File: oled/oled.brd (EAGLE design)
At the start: 35.9 x 35.5 mm, 3 parts

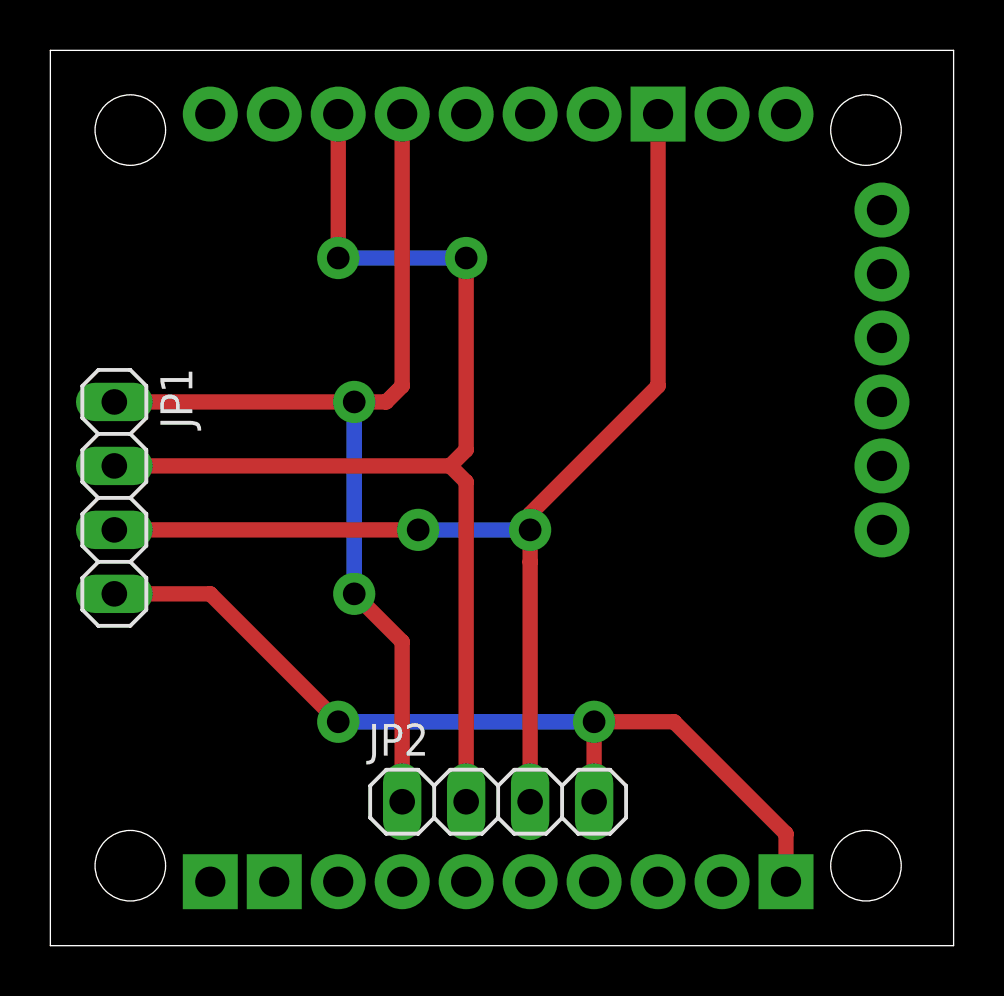
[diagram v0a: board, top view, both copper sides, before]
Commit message: Improve oled board
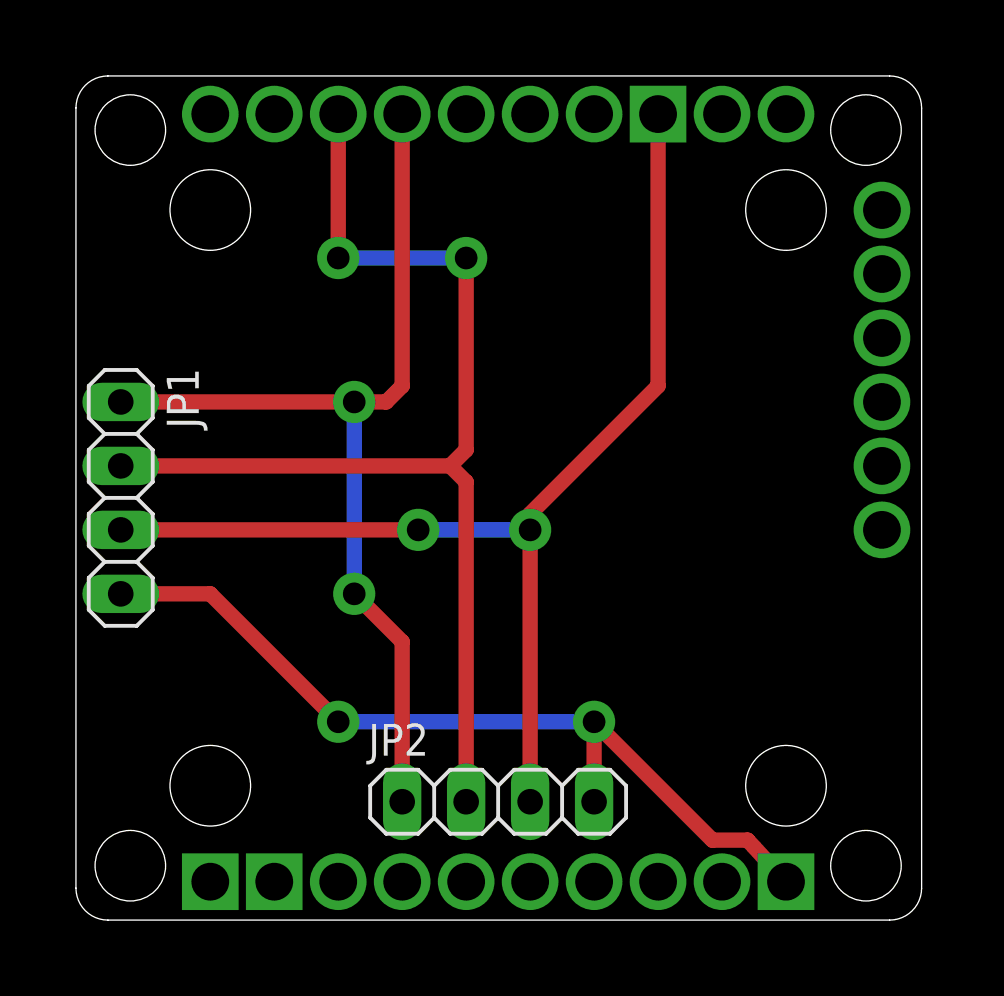
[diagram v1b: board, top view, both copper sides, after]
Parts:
- moved JP1 0.25 mm to (2.79, 17.8)
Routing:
- net +3V3: track 35.7 -> 34.4 mm
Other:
- board size 35.9 x 35.5 mm -> 33.6 x 33.5 mm
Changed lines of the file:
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@@
 <setting verticaltext="up"/>
 </settings>
-<grid distance="0.1" unitdist="inch" unit="inch" style="lines" multiple="1" display="yes" altdistance="0.025" altunitdist="inch" altunit="inch"/>
+<grid distance="0.05" unitdist="inch" unit="inch" style="lines" multiple="1" display="yes" altdistance="0.005" altunitdist="inch" altunit="inch"/>
 <layers>
 <layer number="1" name="Top" color="4" fill="1" visible="yes" active="yes"/>
@@
 <layer number="48" name="Document" color="7" fill="1" visible="yes" active="yes"/>
 <layer number="49" name="Reference" color="7" fill="1" visible="yes" active="yes"/>
+<layer number="50" name="dxf" color="7" fill="1" visible="no" active="no"/>
 <layer number="51" name="tDocu" color="7" fill="1" visible="yes" active="yes"/>
 <layer number="52" name="bDocu" color="7" fill="1" visible="yes" active="yes"/>
+<layer number="53" name="tGND_GNDA" color="7" fill="9" visible="no" active="no"/>
+<layer number="54" name="bGND_GNDA" color="1" fill="9" visible="no" active="no"/>
+<layer number="56" name="wert" color="7" fill="1" visible="no" active="no"/>
 <layer number="90" name="Modules" color="5" fill="1" visible="no" active="no"/>
 <layer number="91" name="Nets" color="2" fill="1" visible="no" active="no"/>
@@
 <layer number="97" name="Info" color="7" fill="1" visible="no" active="no"/>
 <layer number="98" name="Guide" color="6" fill="1" visible="no" active="no"/>
+<layer number="100" name="Muster" color="7" fill="1" visible="no" active="no"/>
+<layer number="101" name="Patch_Top" color="12" fill="4" visible="yes" active="yes"/>
+<layer number="102" name="Vscore" color="7" fill="1" visible="yes" active="yes"/>
+<layer number="103" name="tMap" color="7" fill="1" visible="yes" active="yes"/>
+<layer number="104" name="Name" color="7" fill="1" visible="yes" active="yes"/>
+<layer number="105" name="tPlate" color="7" fill="1" visible="yes" active="yes"/>
+<layer number="106" name="bPlate" color="7" fill="1" visible="yes" active="yes"/>
+<layer number="107" name="Crop" color="7" fill="1" visible="yes" active="yes"/>
+<layer number="116" name="Patch_BOT" color="9" fill="4" visible="yes" active="yes"/>
+<layer number="121" name="_tsilk" color="7" fill="1" visible="yes" active="yes"/>
+<layer number="122" name="_bsilk" color="7" fill="1" visible="yes" active="yes"/>
+<layer number="125" name="_tNames" color="7" fill="1" visible="yes" active="yes"/>
+<layer number="144" name="Drill_legend" color="7" fill="1" visible="yes" active="yes"/>
+<layer number="151" name="HeatSink" color="7" fill="1" visible="yes" active="yes"/>
+<layer number="200" name="200bmp" color="1" fill="10" visible="yes" active="yes"/>
+<layer number="201" name="201bmp" color="2" fill="1" visible="no" active="no"/>
+<layer number="202" name="202bmp" color="3" fill="1" visible="no" active="no"/>
+<layer number="203" name="203bmp" color="4" fill="10" visible="yes" active="yes"/>
+<layer number="204" name="204bmp" color="5" fill="10" visible="yes" active="yes"/>
+<layer number="205" name="205bmp" color="6" fill="10" visible="yes" active="yes"/>
+<layer number="206" name="206bmp" color="7" fill="10" visible="yes" active="yes"/>
+<layer number="207" name="207bmp" color="8" fill="10" visible="yes" active="yes"/>
+<layer number="208" name="208bmp" color="9" fill="10" visible="yes" active="yes"/>
+<layer number="209" name="209bmp" color="7" fill="1" visible="yes" active="yes"/>
+<layer number="210" name="210bmp" color="7" fill="1" visible="yes" active="yes"/>
+<layer number="211" name="211bmp" color="7" fill="1" visible="yes" active="yes"/>
+<layer number="212" name="212bmp" color="7" fill="1" visible="yes" active="yes"/>
+<layer number="213" name="213bmp" color="7" fill="1" visible="yes" active="yes"/>
+<layer number="214" name="214bmp" color="7" fill="1" visible="yes" active="yes"/>
+<layer number="215" name="215bmp" color="7" fill="1" visible="yes" active="yes"/>
+<layer number="216" name="216bmp" color="7" fill="1" visible="yes" active="yes"/>
+<layer number="250" name="Descript" color="3" fill="1" visible="no" active="no"/>
+<layer number="251" name="SMDround" color="12" fill="11" visible="no" active="no"/>
+<layer number="254" name="cooling" color="7" fill="1" visible="yes" active="yes"/>
 </layers>
 <board>
 <plain>
-<wire x1="0" y1="0" x2="35.865" y2="0" width="0" layer="20"/>
-<wire x1="35.865" y1="0" x2="35.865" y2="35.55" width="0" layer="20"/>
-<wire x1="35.865" y1="35.55" x2="0" y2="35.55" width="0" layer="20"/>
-<wire x1="0" y1="35.55" x2="0" y2="0" width="0" layer="20"/>
+<wire x1="2.286" y1="1.016" x2="33.325" y2="1.016" width="0" layer="20"/>
+<wire x1="33.325" y1="1.016" x2="34.595" y2="2.286" width="0" layer="20" curve="90"/>
+<wire x1="34.595" y1="2.286" x2="34.595" y2="33.264" width="0" layer="20"/>
+<wire x1="34.595" y1="33.264" x2="33.325" y2="34.534" width="0" layer="20" curve="90"/>
+<wire x1="33.325" y1="34.534" x2="2.286" y2="34.534" width="0" layer="20"/>
+<wire x1="2.286" y1="34.534" x2="1.016" y2="33.264" width="0" layer="20" curve="90"/>
+<wire x1="1.016" y1="33.264" x2="1.016" y2="2.286" width="0" layer="20"/>
+<wire x1="1.016" y1="2.286" x2="2.286" y2="1.016" width="0" layer="20" curve="90"/>
+<hole x="29.21" y="6.35" drill="3.2"/>
+<hole x="6.35" y="6.35" drill="3.2"/>
+<hole x="29.21" y="29.21" drill="3.2"/>
+<hole x="6.35" y="29.21" drill="3.2"/>
 </plain>
 <attributes>
@@
 <elements>
 <element name="OLED/I2C" library="ESPstack" package="ESP-BOARD" value="ESP-BOARD" x="24.13" y="19.05"/>
-<element name="JP1" library="pinhead" package="1X04" value="" x="2.54" y="17.78" rot="R270"/>
+<element name="JP1" library="pinhead" package="1X04" value="" x="2.794" y="17.78" rot="R270"/>
 <element name="JP2" library="pinhead" package="1X04" value="" x="17.78" y="5.715"/>
 </elements>
@@
 <contactref element="JP1" pad="4"/>
 <contactref element="JP2" pad="4"/>
-<wire x1="2.54" y1="13.97" x2="6.35" y2="13.97" width="0.6096" layer="1"/>
+<wire x1="2.794" y1="13.97" x2="6.35" y2="13.97" width="0.6096" layer="1"/>
 <wire x1="6.35" y1="13.97" x2="11.43" y2="8.89" width="0.6096" layer="1"/>
 <via x="11.43" y="8.89" extent="1-16" drill="0.9" diameter="1.6764"/>
@@
 <via x="21.59" y="8.89" extent="1-16" drill="0.9" diameter="1.6764"/>
 <wire x1="21.59" y1="8.89" x2="21.59" y2="5.715" width="0.6096" layer="1"/>
-<wire x1="29.21" y1="2.54" x2="29.21" y2="4.445" width="0.6096" layer="1"/>
-<wire x1="29.21" y1="4.445" x2="24.765" y2="8.89" width="0.6096" layer="1"/>
-<wire x1="24.765" y1="8.89" x2="21.59" y2="8.89" width="0.6096" layer="1"/>
+<wire x1="29.21" y1="2.54" x2="27.686" y2="4.191" width="0.6096" layer="1"/>
+<wire x1="27.686" y1="4.191" x2="26.289" y2="4.191" width="0.6096" layer="1"/>
+<wire x1="26.289" y1="4.191" x2="21.59" y2="8.89" width="0.6096" layer="1"/>
 </signal>
 <signal name="GND">
@@
 <contactref element="JP1" pad="3"/>
 <contactref element="OLED/I2C" pad="GND"/>
-<wire x1="19.05" y1="5.715" x2="19.05" y2="15.24" width="0.6096" layer="1"/>
+<wire x1="19.05" y1="5.715" x2="19.05" y2="16.51" width="0.6096" layer="1"/>
 <wire x1="19.05" y1="16.51" x2="19.05" y2="17.145" width="0.6096" layer="1"/>
 <wire x1="19.05" y1="17.145" x2="24.13" y2="22.225" width="0.6096" layer="1"/>
 <wire x1="24.13" y1="22.225" x2="24.13" y2="33.02" width="0.6096" layer="1"/>
-<wire x1="2.54" y1="16.51" x2="14.605" y2="16.51" width="0.6096" layer="1"/>
+<wire x1="2.794" y1="16.51" x2="14.605" y2="16.51" width="0.6096" layer="1"/>
 <via x="14.605" y="16.51" extent="1-16" drill="0.9" diameter="1.6764"/>
 <wire x1="14.605" y1="16.51" x2="19.05" y2="16.51" width="0.6096" layer="16"/>
 <via x="19.05" y="16.51" extent="1-16" drill="0.9" diameter="1.6764"/>
-<wire x1="19.05" y1="16.51" x2="19.05" y2="15.24" width="0.6096" layer="1"/>
 </signal>
 <signal name="SDA">
@@
 <wire x1="12.065" y1="13.97" x2="12.065" y2="21.59" width="0.6096" layer="16"/>
 <via x="12.065" y="21.59" extent="1-16" drill="0.9" diameter="1.6764"/>
-<wire x1="12.065" y1="21.59" x2="2.54" y2="21.59" width="0.6096" layer="1"/>
+<wire x1="12.065" y1="21.59" x2="2.794" y2="21.59" width="0.6096" layer="1"/>
 </signal>
 <signal name="SCL">
@@
 <contactref element="JP2" pad="2"/>
 <contactref element="OLED/I2C" pad="GPIO5"/>
-<wire x1="2.54" y1="19.05" x2="15.875" y2="19.05" width="0.6096" layer="1"/>
+<wire x1="2.794" y1="19.05" x2="15.875" y2="19.05" width="0.6096" layer="1"/>
 <wire x1="15.875" y1="19.05" x2="16.51" y2="18.415" width="0.6096" layer="1"/>
 <wire x1="16.51" y1="18.415" x2="16.51" y2="5.715" width="0.6096" layer="1"/>
